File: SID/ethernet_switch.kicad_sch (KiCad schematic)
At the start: 0 parts

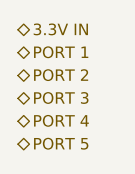
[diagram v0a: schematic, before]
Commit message: Feat(SID): basically complete
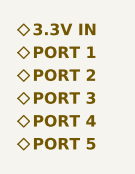
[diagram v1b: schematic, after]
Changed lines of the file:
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@@
-(kicad_sch (version 20230819) (generator eeschema)
-  (paper "A4")
-  (hierarchical_label "PORT 1" (shape bidirectional) (at 109.22 93.98 0) (fields_autoplaced)
-    (effects (font (size 1.27 1.27)) (justify left))
-  )
-  (hierarchical_label "PORT 3" (shape bidirectional) (at 109.22 99.06 0) (fields_autoplaced)
-    (effects (font (size 1.27 1.27)) (justify left))
-  )
-  (hierarchical_label "PORT 5" (shape bidirectional) (at 109.22 104.14 0) (fields_autoplaced)
-    (effects (font (size 1.27 1.27)) (justify left))
-  )
-  (hierarchical_label "PORT 2" (shape bidirectional) (at 109.22 96.52 0) (fields_autoplaced)
-    (effects (font (size 1.27 1.27)) (justify left))
-  )
-  (hierarchical_label "3.3V IN" (shape bidirectional) (at 109.22 91.44 0) (fields_autoplaced)
-    (effects (font (size 1.27 1.27)) (justify left))
-  )
-  (hierarchical_label "PORT 4" (shape bidirectional) (at 109.22 101.6 0) (fields_autoplaced)
-    (effects (font (size 1.27 1.27)) (justify left))
-  )
+(kicad_sch
+	(version 20240101)
+	(generator "eeschema")
+	(generator_version "8.99")
+	(paper "A4")
+	(hierarchical_label "PORT 1"
+		(shape bidirectional)
+		(at 109.22 93.98 0)
+		(fields_autoplaced yes)
+		(effects
+			(font
+				(face "JetBrains Mono")
+				(size 1.27 1.27)
+				(thickness 0.254)
+				(bold yes)
+			)
+			(justify left)
+		)
+	)
+	(hierarchical_label "PORT 3"
+		(shape bidirectional)
+		(at 109.22 99.06 0)
+		(fields_autoplaced yes)
+		(effects
+			(font
+				(face "JetBrains Mono")
+				(size 1.27 1.27)
+				(thickness 0.254)
+				(bold yes)
+			)
+			(justify left)
+		)
+	)
+	(hierarchical_label "PORT 5"
+		(shape bidirectional)
+		(at 109.22 104.14 0)
+		(fields_autoplaced yes)
+		(effects
+			(font
+				(face "JetBrains Mono")
+				(size 1.27 1.27)
+				(thickness 0.254)
+				(bold yes)
+			)
+			(justify left)
+		)
+	)
+	(hierarchical_label "PORT 2"
+		(shape bidirectional)
+		(at 109.22 96.52 0)
+		(fields_autoplaced yes)
+		(effects
+			(font
+				(face "JetBrains Mono")
+				(size 1.27 1.27)
+				(thickness 0.254)
+				(bold yes)
+			)
+			(justify left)
+		)
+	)
+	(hierarchical_label "3.3V IN"
+		(shape bidirectional)
+		(at 109.22 91.44 0)
+		(fields_autoplaced yes)
+		(effects
+			(font
+				(face "JetBrains Mono")
+				(size 1.27 1.27)
+				(thickness 0.254)
+				(bold yes)
+			)
+			(justify left)
+		)
+	)
+	(hierarchical_label "PORT 4"
+		(shape bidirectional)
+		(at 109.22 101.6 0)
+		(fields_autoplaced yes)
+		(effects
+			(font
+				(face "JetBrains Mono")
+				(size 1.27 1.27)
+				(thickness 0.254)
+				(bold yes)
+			)
+			(justify left)
+		)
+	)
 )
